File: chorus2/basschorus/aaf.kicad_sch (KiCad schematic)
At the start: 7 parts, among them U4 TL074

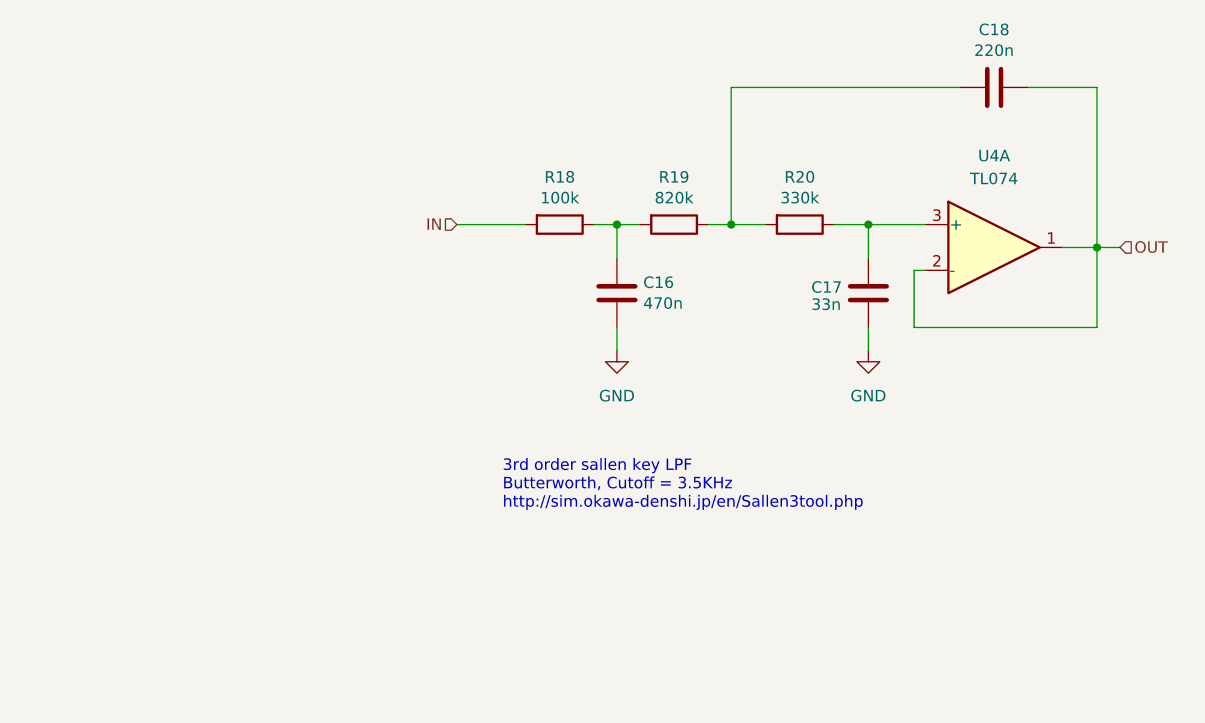
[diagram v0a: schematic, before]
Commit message: update filters
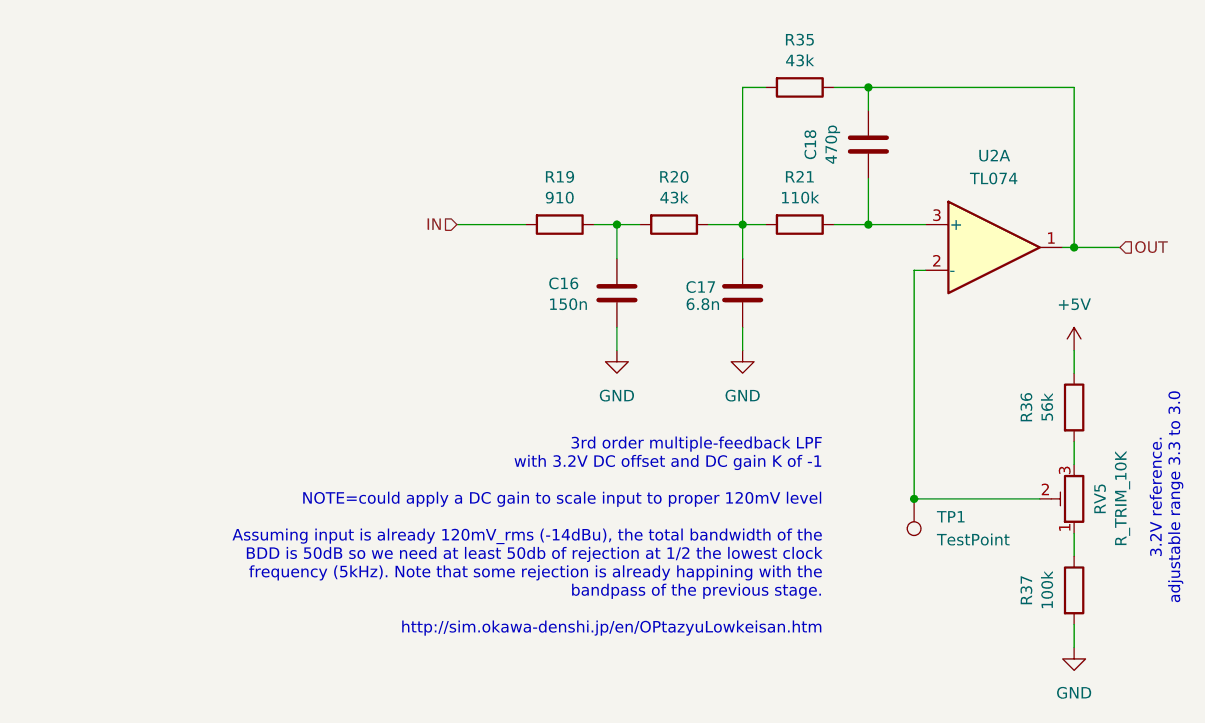
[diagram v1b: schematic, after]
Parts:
- added R35: 43k, kicad-legacy/kicad-footprints/Resistor_THT.pretty:R_Axial_DIN0204_L3.6mm_D1.6mm_P2.54mm_Vertical, symbol Device:R
- added R36: 56k, kicad-legacy/kicad-footprints/Resistor_THT.pretty:R_Axial_DIN0204_L3.6mm_D1.6mm_P2.54mm_Vertical, symbol Device:R
- added R37: 100k, kicad-legacy/kicad-footprints/Resistor_THT.pretty:R_Axial_DIN0204_L3.6mm_D1.6mm_P2.54mm_Vertical, symbol Device:R
- added RV5: R_TRIM_10K, kicad-legacy/Potentiometers.pretty:Potentiometer_Trimmer_Bourns_3296W, symbol Device:R_Potentiometer_Trim
- added TP1: TestPoint, symbol Connector:TestPoint
- C16: value 470n -> 150n
- C17: value 33n -> 6.8n
- C18: value 220n -> 470p
- R19: renamed from R18; value 100k -> 910
- R20: renamed from R19; value 820k -> 43k
- R21: renamed from R20; value 330k -> 110k
- renumbered U4 to U2
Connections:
- net GND: now also R37.2
- net OUT: now also R35.1; no longer U2.2 (-)
- net at R21.1, U2.3 (+): now also C18.2; no longer C17.2
- net at R20.1, R21.2: now also C17.2, R35.2; no longer C18.2
- new net: R36.2, RV5.3
- new net: R37.1, RV5.1
- new net: RV5.2, TP1.1, U2.2 (-)
- new net +5V: R36.1
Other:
- note added: "3.2V reference. adjustable range 3.3 to 3.0"
- note added: "3rd order multiple-feedback LPF with 3.2V DC offset and DC gain K of -1 NOTE=could apply a DC gain to scale input to proper 120mV level Assuming input is already 120mV_rms (-14dBu), the total bandwidth of the BDD is 50dB so we need at least 50db of rejection at 1/2 the lowest clock frequency (5kHz). Note that some rejection is already happining with the bandpass of the previous stage. http://sim.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"
- note removed: "3rd order sallen key LPF Butterworth, Cutoff = 3.5KHz http://sim.okawa-denshi.jp/en/Sallen3tool.php"
- moved on the sheet: C17, C18
